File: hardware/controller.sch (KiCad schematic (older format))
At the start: 1 part

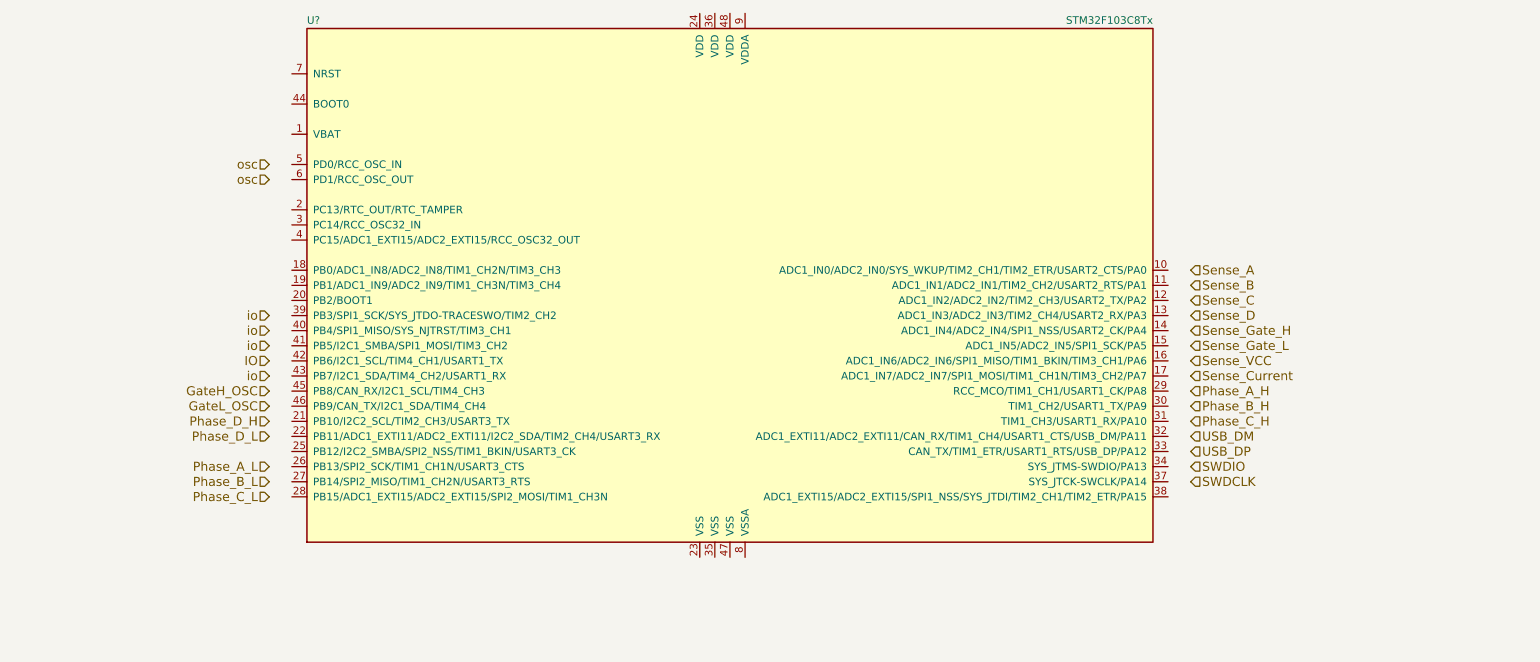
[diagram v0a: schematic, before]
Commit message: power, mcu
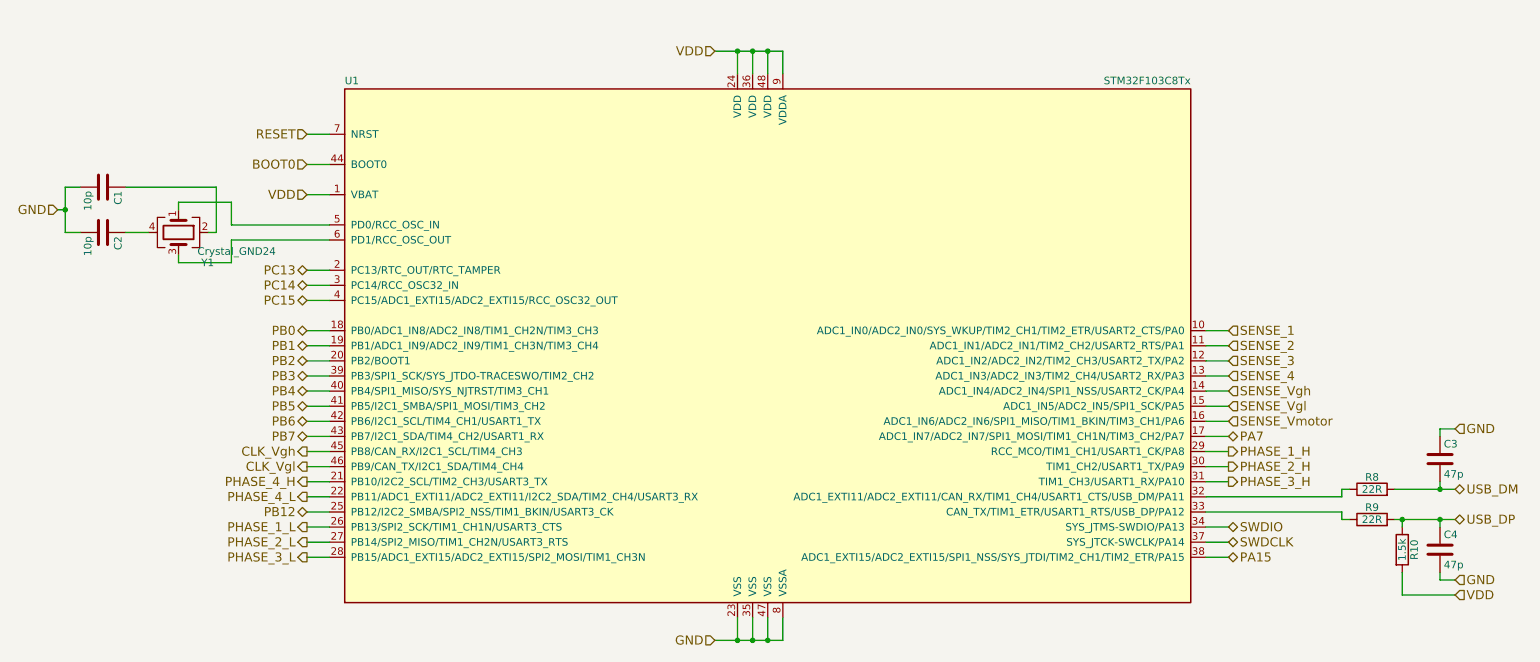
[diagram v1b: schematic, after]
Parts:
- added C1, C2: 10p, Capacitors_SMD:C_0603, symbol C
- added C3, C4: 47p, Capacitors_SMD:C_0603, symbol C
- added R10: 1.5k, Resistors_SMD:R_0603, symbol R
- added R8, R9: 22R, Resistors_SMD:R_0603, symbol R
- added Y1: Crystal_GND24, Crystals:Crystal_SMD_3225-4pin_3.2x2.5mm, symbol Crystal_GND24
- gave numbers to parts that had none: 1
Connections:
- net SWDCLK: now also U1.37 (SYS_JTCK-SWCLK/PA14)
- net SWDIO: now also U1.34 (SYS_JTMS-SWDIO/PA13)
- net USB_DM: now also C3.2, R8.2
- net USB_DP: now also C4.1, R10.1, R9.2
- net VDD: now reaches U1.1 (VBAT)
- net VDD: now also U1.24 (VDD), U1.36 (VDD), U1.48 (VDD), U1.9 (VDDA), R10.2
- net SENSE_1: now reaches U1.10 (ADC1_IN0/ADC2_IN0/SYS_WKUP/TIM2_CH1/TIM2_ETR/USART2_CTS/PA0)
- net SENSE_2: now reaches U1.11 (ADC1_IN1/ADC2_IN1/TIM2_CH2/USART2_RTS/PA1)
- net SENSE_3: now reaches U1.12 (ADC1_IN2/ADC2_IN2/TIM2_CH3/USART2_TX/PA2)
- net SENSE_4: now reaches U1.13 (ADC1_IN3/ADC2_IN3/TIM2_CH4/USART2_RX/PA3)
- net SENSE_Vgh: now reaches U1.14 (ADC1_IN4/ADC2_IN4/SPI1_NSS/USART2_CK/PA4)
- net SENSE_Vgl: now reaches U1.15 (ADC1_IN5/ADC2_IN5/SPI1_SCK/PA5)
- net SENSE_Vmotor: now reaches U1.16 (ADC1_IN6/ADC2_IN6/SPI1_MISO/TIM1_BKIN/TIM3_CH1/PA6)
- net PA7: now reaches U1.17 (ADC1_IN7/ADC2_IN7/SPI1_MOSI/TIM1_CH1N/TIM3_CH2/PA7)
- net PB0: now reaches U1.18 (PB0/ADC1_IN8/ADC2_IN8/TIM1_CH2N/TIM3_CH3)
- net PB1: now reaches U1.19 (PB1/ADC1_IN9/ADC2_IN9/TIM1_CH3N/TIM3_CH4)
- net PC13: now reaches U1.2 (PC13/RTC_OUT/RTC_TAMPER)
- net PB2: now reaches U1.20 (PB2/BOOT1)
- net PHASE_4_H: now reaches U1.21 (PB10/I2C2_SCL/TIM2_CH3/USART3_TX)
- net PHASE_4_L: now reaches U1.22 (PB11/ADC1_EXTI11/ADC2_EXTI11/I2C2_SDA/TIM2_CH4/USART3_RX)
- net GND: now reaches U1.23 (VSS)
- net GND: now also U1.35 (VSS), U1.47 (VSS), U1.8 (VSSA), C1.2, C2.2, C3.1, C4.2
- net PB12: now reaches U1.25 (PB12/I2C2_SMBA/SPI2_NSS/TIM1_BKIN/USART3_CK)
- net PHASE_1_L: now reaches U1.26 (PB13/SPI2_SCK/TIM1_CH1N/USART3_CTS)
- net PHASE_2_L: now reaches U1.27 (PB14/SPI2_MISO/TIM1_CH2N/USART3_RTS)
- net PHASE_3_L: now reaches U1.28 (PB15/ADC1_EXTI15/ADC2_EXTI15/SPI2_MOSI/TIM1_CH3N)
- net PHASE_1_H: now reaches U1.29 (RCC_MCO/TIM1_CH1/USART1_CK/PA8)
- net PC14: now reaches U1.3 (PC14/RCC_OSC32_IN)
- net PHASE_2_H: now reaches U1.30 (TIM1_CH2/USART1_TX/PA9)
- net PHASE_3_H: now reaches U1.31 (TIM1_CH3/USART1_RX/PA10)
- net at U1.32 (ADC1_EXTI11/ADC2_EXTI11/CAN_RX/TIM1_CH4/USART1_CTS/USB_DM/PA11): now also R8.1
- net at U1.33 (CAN_TX/TIM1_ETR/USART1_RTS/USB_DP/PA12): now also R9.1
- net PA15: now reaches U1.38 (ADC1_EXTI15/ADC2_EXTI15/SPI1_NSS/SYS_JTDI/TIM2_CH1/TIM2_ETR/PA15)
- net PB3: now reaches U1.39 (PB3/SPI1_SCK/SYS_JTDO-TRACESWO/TIM2_CH2)
- net PC15: now reaches U1.4 (PC15/ADC1_EXTI15/ADC2_EXTI15/RCC_OSC32_OUT)
- net PB4: now reaches U1.40 (PB4/SPI1_MISO/SYS_NJTRST/TIM3_CH1)
- net PB5: now reaches U1.41 (PB5/I2C1_SMBA/SPI1_MOSI/TIM3_CH2)
- net PB6: now reaches U1.42 (PB6/I2C1_SCL/TIM4_CH1/USART1_TX)
- net PB7: now reaches U1.43 (PB7/I2C1_SDA/TIM4_CH2/USART1_RX)
- net BOOT0: now reaches U1.44 (BOOT0)
- net CLK_Vgh: now reaches U1.45 (PB8/CAN_RX/I2C1_SCL/TIM4_CH3)
- net CLK_Vgl: now reaches U1.46 (PB9/CAN_TX/I2C1_SDA/TIM4_CH4)
- net at U1.5 (PD0/RCC_OSC_IN): now also Y1.1
- net at U1.6 (PD1/RCC_OSC_OUT): now also Y1.3
- net RESET: now reaches U1.7 (NRST)
- new net: C1.1, Y1.2
- new net: C2.1, Y1.4
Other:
- moved on the sheet: U1
